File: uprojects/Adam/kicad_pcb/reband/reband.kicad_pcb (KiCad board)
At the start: 2 copper layers, 25 x 30 mm, 11 parts, among them J1 S2B-ZRLFSN, J2 USB4215-03-A, U1 ESP32-C3FH4, U2 AP2112K-3.3TRG1, U3 MAX30009ENA+T, U4 BQ25100YFPR, U5 BNO055, U6 TCR2EF33_LMCT, U7 TCR2EF18_LMCT

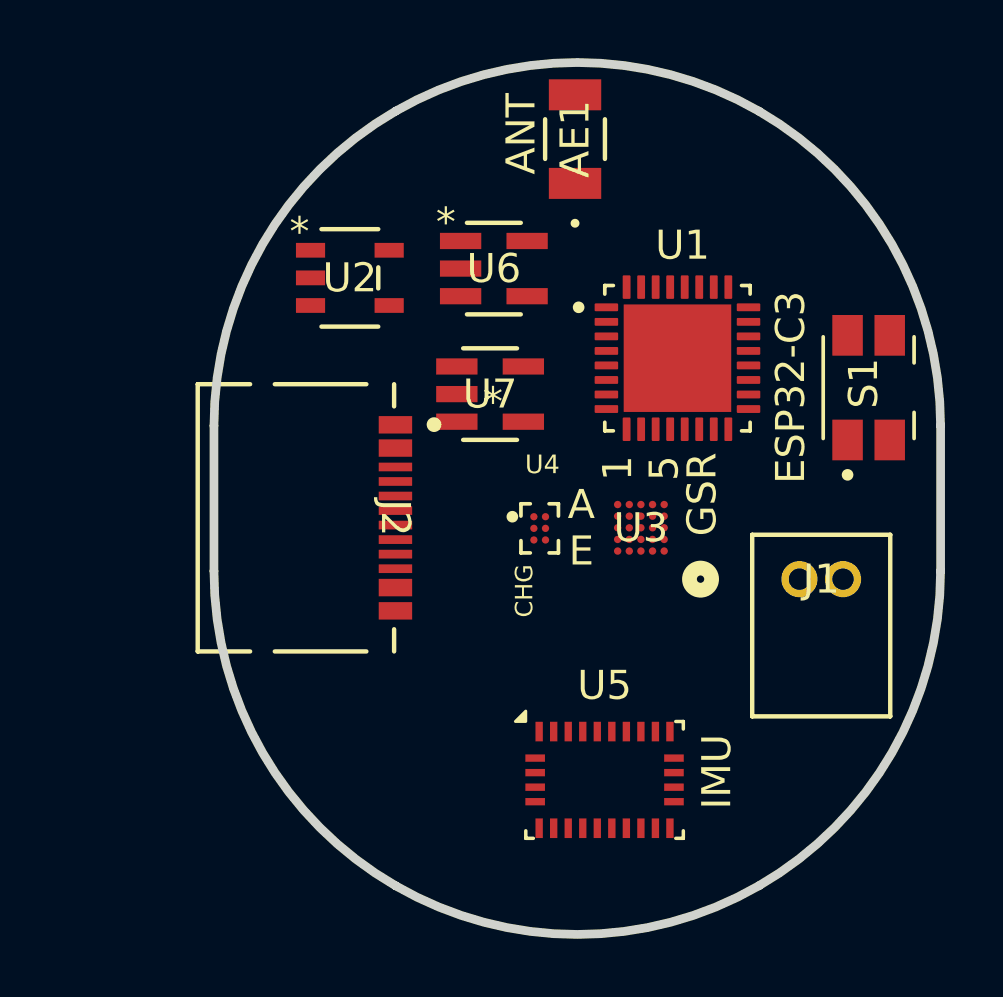
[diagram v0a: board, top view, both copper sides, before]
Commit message: Update 28 May 2026
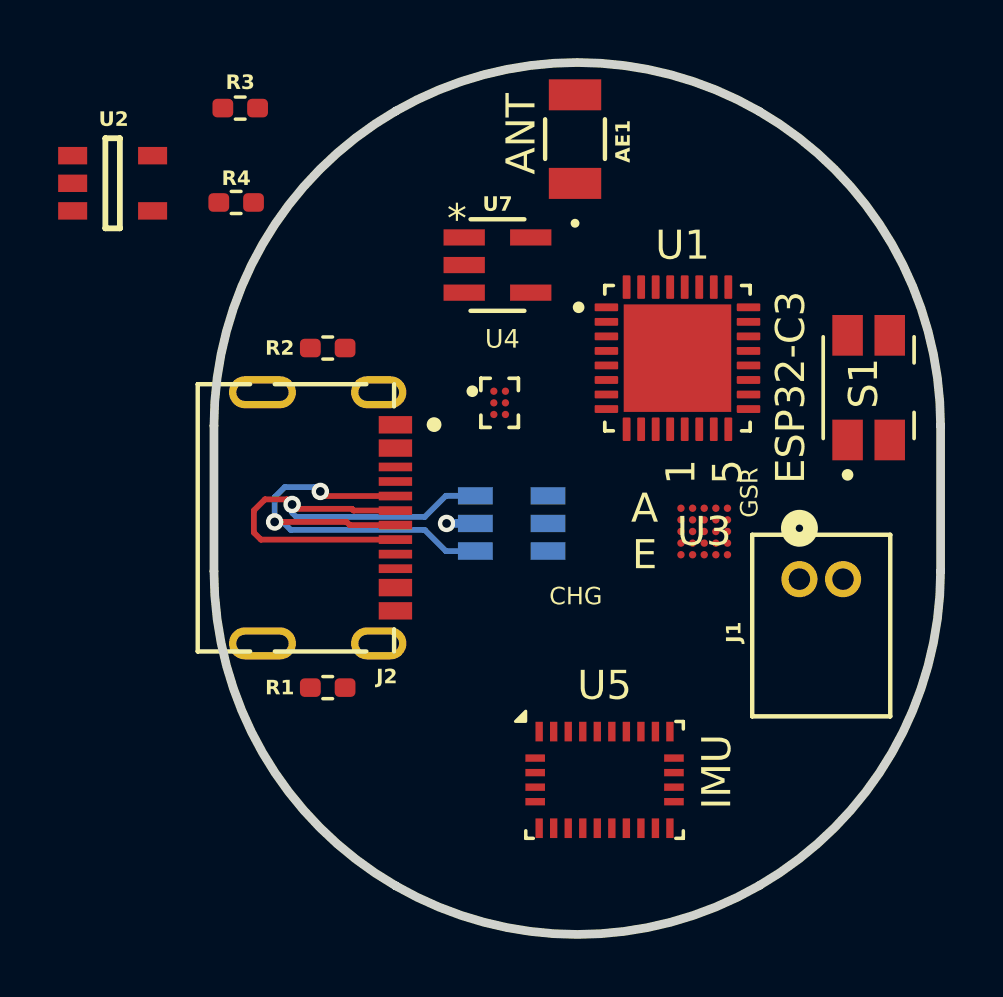
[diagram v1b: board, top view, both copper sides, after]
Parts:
- removed U6: TCR2EF33_LMCT, TCR2EF33_LM_CT:SOT-25 SMV_TOS
- added IC1: USBLC6-2SC6, USBLC6-2SC6:SOT95P280X145-6N, B.Cu at (137.4, 90.1)
- added R1: 5.1K, Resistor_SMD:R_0402_1005Metric_Pad0.72x0.64mm_HandSolder, F.Cu at (131.1, 95.8)
- added R2: 5.1K, Resistor_SMD:R_0402_1005Metric_Pad0.72x0.64mm_HandSolder, F.Cu at (131.1, 84.1)
- added R3: 10K, Resistor_SMD:R_0402_1005Metric_Pad0.72x0.64mm_HandSolder, F.Cu at (128.1, 75.8)
- added R4: 2K7, Resistor_SMD:R_0402_1005Metric_Pad0.72x0.64mm_HandSolder, F.Cu at (127.9, 79.1)
- U2: value AP2112K-3.3TRG1 -> TLV75533PDBVR; footprint AP2112K_3_3TRG1:SOT_RG1_DIO -> TLV75533PDBVR:DBV0005A_N
- moved U2 8.79 mm to (123.7, 78.4)
- moved U4 4.53 mm to (137.0, 86.0)
- moved U7 4.45 mm to (136.9, 81.2)
- moved U3 2.18 mm to (144.0, 90.4)
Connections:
- J2 pad A1/B12: unconnected-(J2-GND-PadA1/B12) -> GND
- J2 pad A4/B9: unconnected-(J2-VBUS-PadA4/B9) -> +5V
- J2 pad A5: unconnected-(J2-CC1-PadA5) -> Net-(J2-CC1)
- J2 pad A6: unconnected-(J2-DP1-PadA6) -> /USB_D+
- J2 pad A7: unconnected-(J2-DN1-PadA7) -> /USB_D-
- J2 pad B1/A12: unconnected-(J2-GND-PadB1/A12) -> GND
- J2 pad B4/A9: unconnected-(J2-VBUS-PadB4/A9) -> +5V
- J2 pad B5: unconnected-(J2-CC2-PadB5) -> Net-(J2-CC2)
- J2 pad B6: unconnected-(J2-DP2-PadB6) -> /USB_D+
- J2 pad B7: unconnected-(J2-DN2-PadB7) -> /USB_D-
- U4 pad A2: unconnected-(U4-IN-PadA2) -> +5V
- U4 pad B2: unconnected-(U4-ISET-PadB2) -> Net-(U4-ISET)
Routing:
- net /USB_D+: track 0.00 -> 17.9 mm, vias 0 -> 1
- net /USB_D-: track 0.00 -> 16.8 mm, vias 0 -> 2
- net GND: track 0.00 -> 1.08 mm, vias 0 -> 1
